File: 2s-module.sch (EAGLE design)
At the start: 34 parts, among them J1 CQ-USB-C16PSMT01, Q1 IRFR9020A, U1 MCP4725, U2 PC817XI, U3 LM393DR, U4 MICROCHIP_MIC5219-3_3YM5-TRMI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

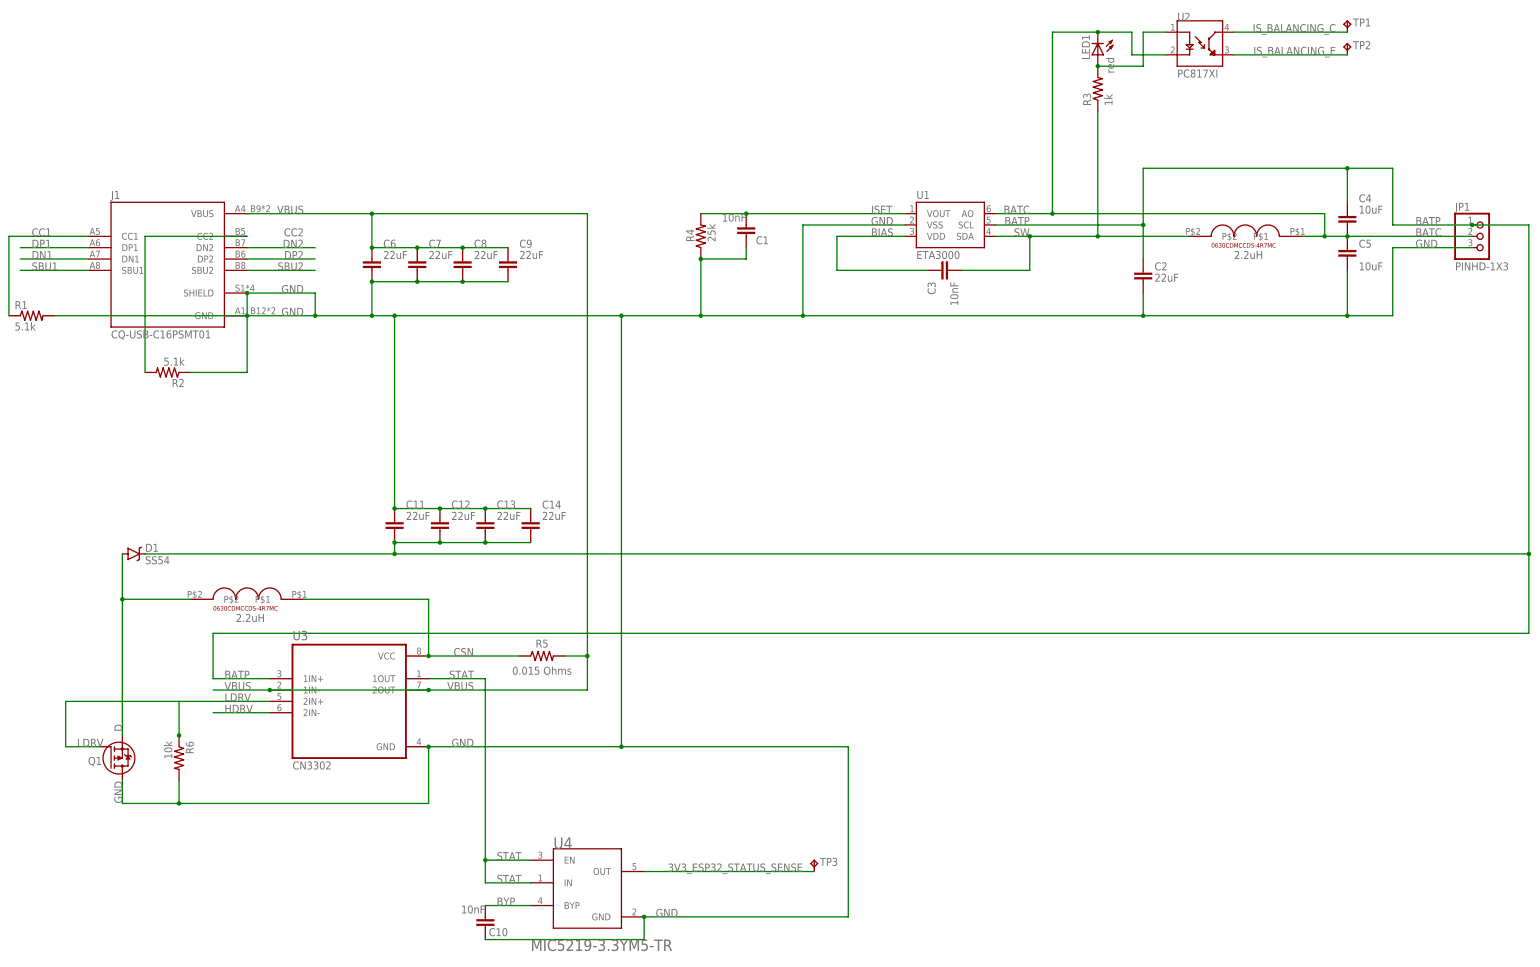
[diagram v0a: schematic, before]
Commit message: fix some parts in sch
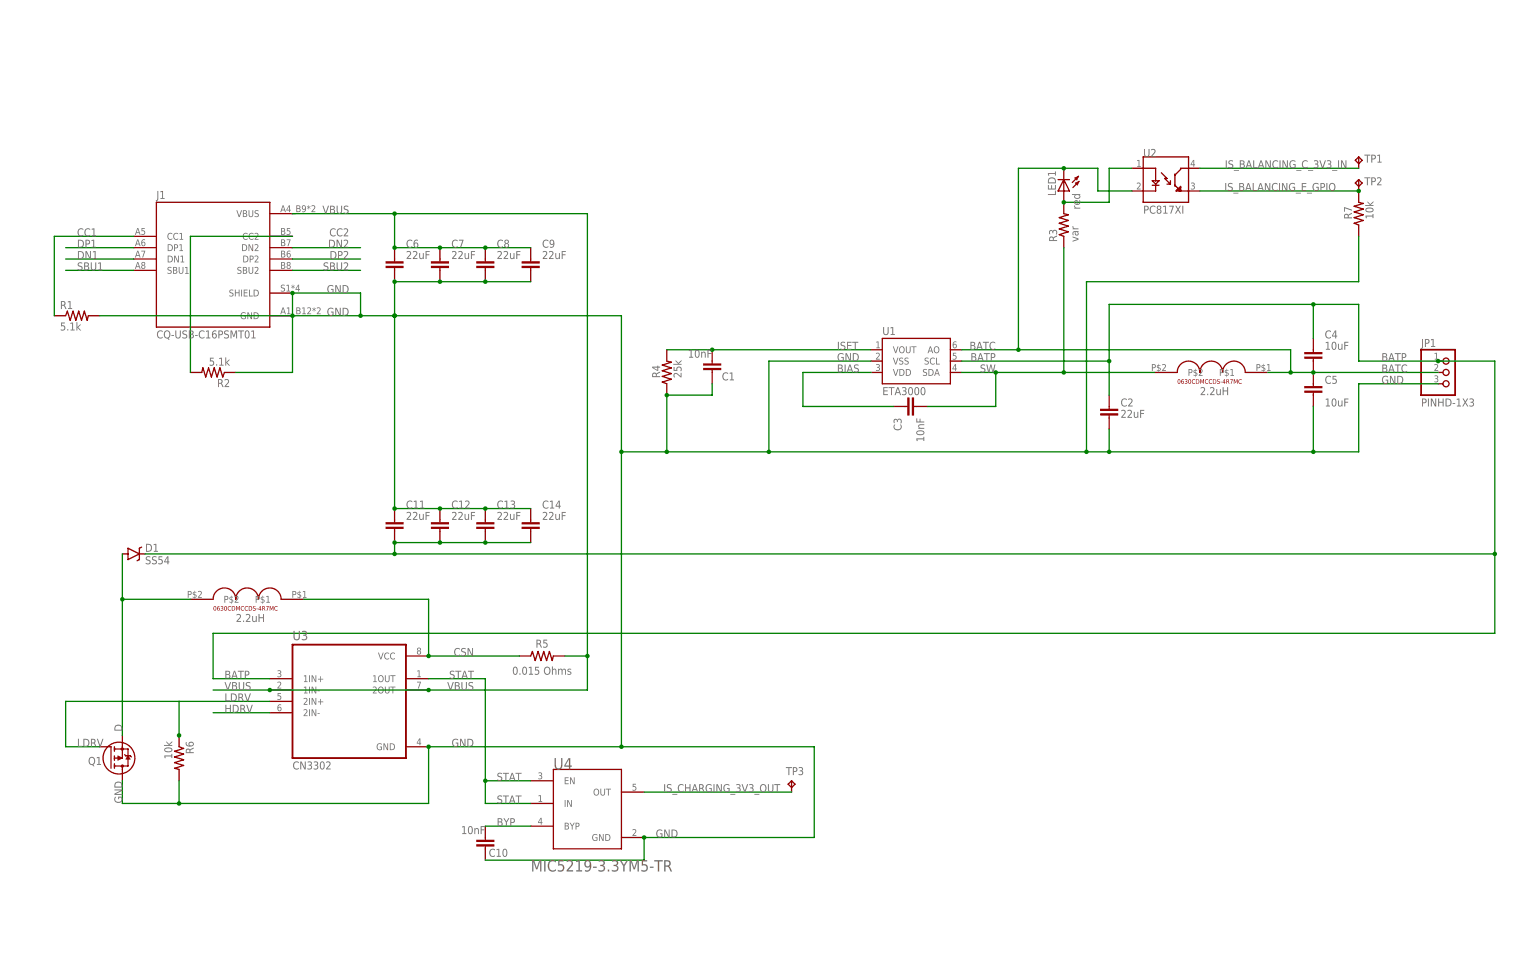
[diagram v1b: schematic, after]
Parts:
- added R7: 10k, resistor:R-US_R0603
- R3: value 1k -> var
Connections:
- net 3V3_ESP32_STATUS_SENSE renamed IS_CHARGING_3V3_OUT
- net IS_BALANCING_C renamed IS_BALANCING_C_3V3_IN
- removed net IS_BALANCING_E: TP2.TP, U2.ET
- new net IS_BALANCING_E_GPIO: R7.2, TP2.TP, U2.ET
- net GND: now also R7.1
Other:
- moved on the sheet: C1, C10, C2, C3, C4, C5, C6, C7, C8, C9, J1, JP1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
